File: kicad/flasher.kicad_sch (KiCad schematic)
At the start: 31 parts, among them U8 FT232H, U9 93LC56BT-I/OT

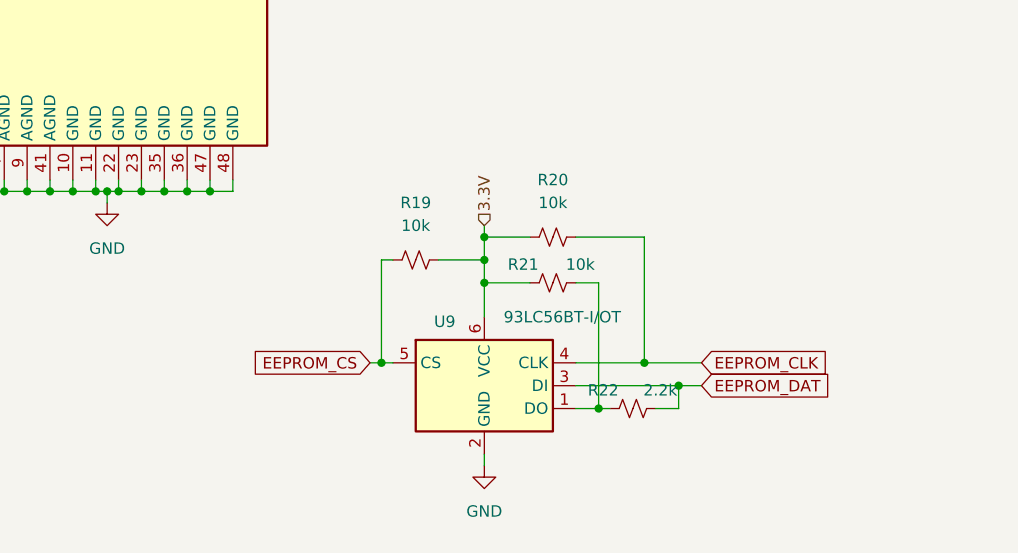
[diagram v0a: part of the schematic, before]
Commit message: update bom and journal
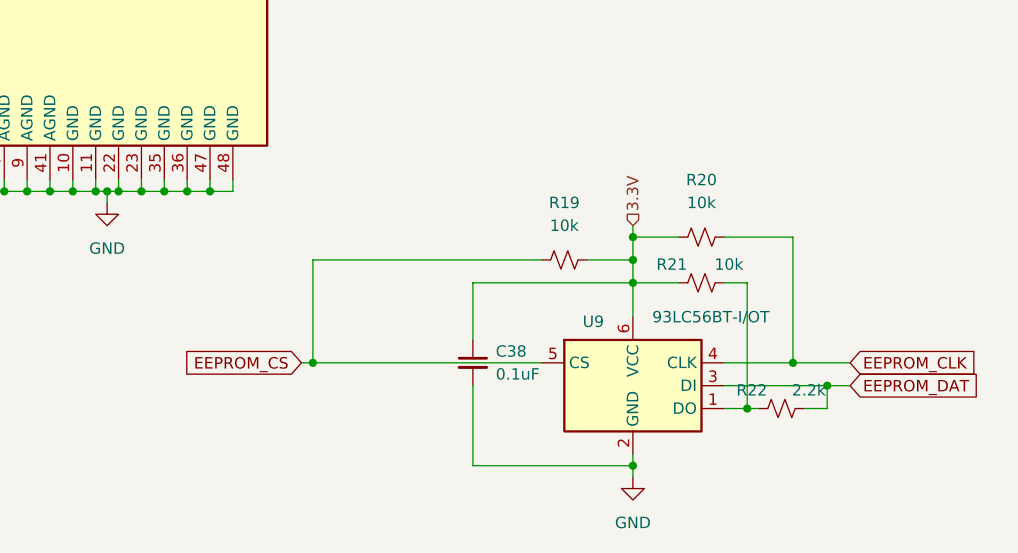
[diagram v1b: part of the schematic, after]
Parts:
- added C38: 0.1uF, Capacitor_SMD:C_0402_1005Metric, symbol Device:C_Small
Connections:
- net 3.3V: now also C38.1
- net GND: now also C38.2
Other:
- moved on the sheet: R19, R20, R21, R22, U9
